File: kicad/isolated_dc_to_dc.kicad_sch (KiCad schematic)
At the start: 23 parts, among them U1001 LM25184NGUR, U1002 750313445

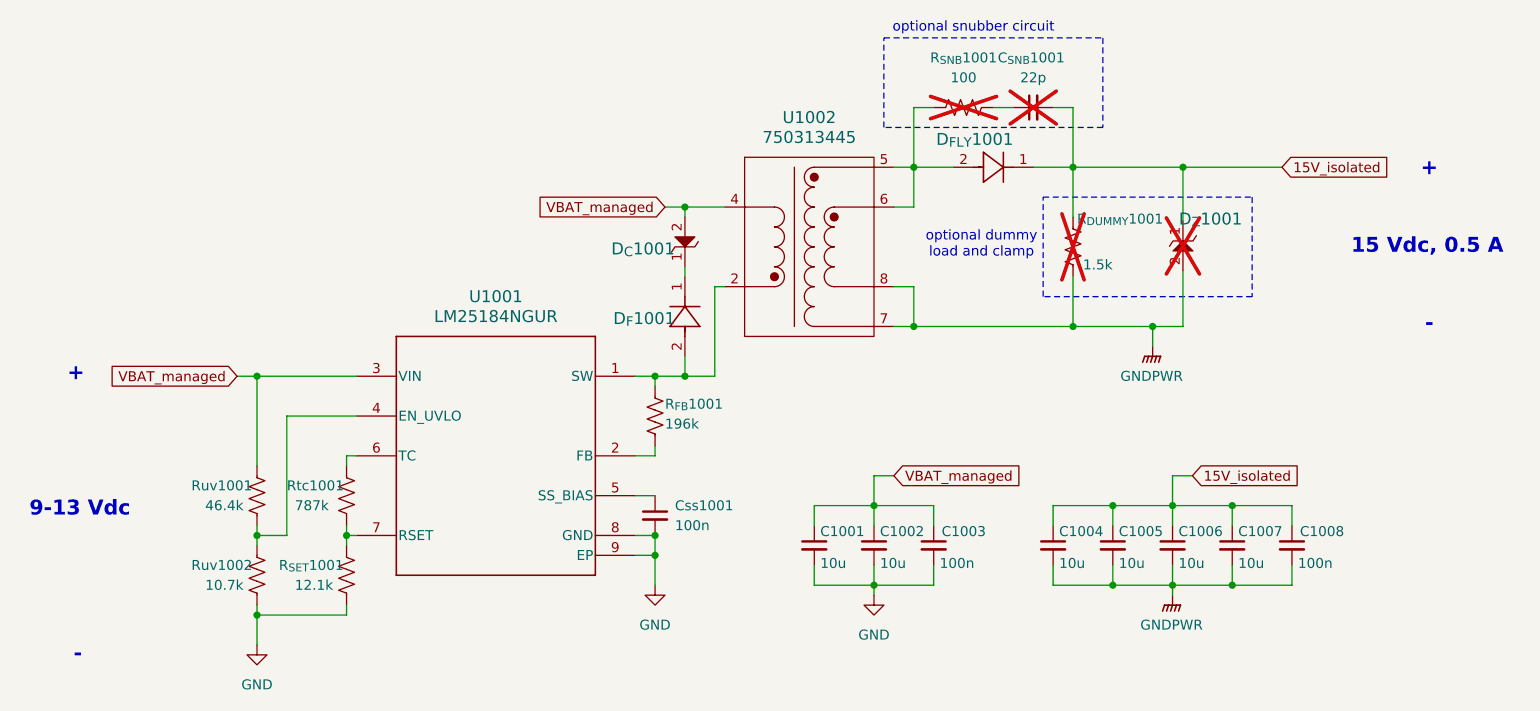
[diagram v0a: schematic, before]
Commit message: kicad
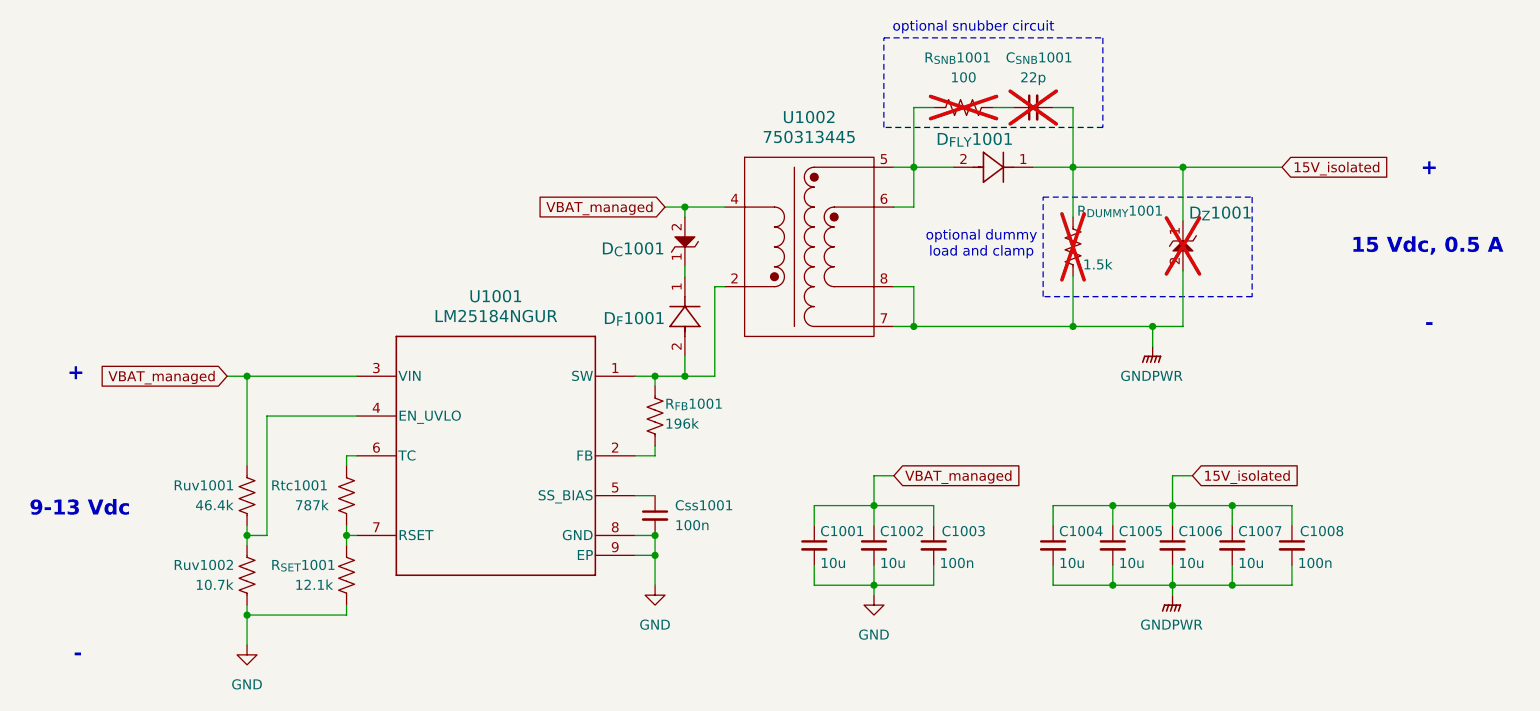
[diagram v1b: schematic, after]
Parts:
- D_{C}1001, D_{Z}1001: footprint zener_PDZVTR9.1B:DIO_PDZVTFT_ROM -> DIO_PDZVTFT_ROM
- D_{FLY}1001, D_{F}1001: footprint schottky_SK510A-LTP:SMADO-214AC_LEAD-FRAME_MCC -> SMADO-214AC_LEAD-FRAME_MCC
- U1001: footprint dc_to_dc_LM25184NGUR:NGU0008C-IPC_A -> NGU0008C-IPC_A
- U1002: footprint transformer_750313445:SOIC_13445_WRE -> SOIC_13445_WRE
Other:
- moved on the sheet: Ruv1001, Ruv1002
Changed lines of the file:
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@@
 	(paper "A4")
-	(junction
-		(at 109.22 96.52)
-		(diameter 0)
-		(color 0 0 0 0)
-	)
-	(junction
-		(at 109.22 66.04)
-		(diameter 0)
-		(color 0 0 0 0)
-	)
 	(junction
 		(at 233.68 92.71)
@@
 	)
 	(junction
+		(at 107.95 96.52)
+		(diameter 0)
+		(color 0 0 0 0)
+	)
+	(junction
 		(at 227.3899 39.37)
+		(diameter 0)
+		(color 0 0 0 0)
+	)
+	(junction
+		(at 107.95 66.04)
 		(diameter 0)
 		(color 0 0 0 0)
@@
 	)
 	(junction
-		(at 109.22 86.36)
-		(diameter 0)
-		(color 0 0 0 0)
-	)
-	(junction
 		(at 187.96 92.71)
 		(diameter 0)
@@
 	)
 	(junction
+		(at 107.95 86.36)
+		(diameter 0)
+		(color 0 0 0 0)
+	)
+	(junction
 		(at 160.02 86.36)
 		(diameter 0)
@@
 	(wire
 		(pts
-			(xy 113.03 86.36) (xy 109.22 86.36)
-		)
-		(stroke
-			(width 0)
-			(type default)
-		)
-	)
-	(wire
-		(pts
 			(xy 160.02 67.31) (xy 160.02 66.04)
 		)
@@
 	(wire
 		(pts
-			(xy 109.22 66.04) (xy 121.92 66.04)
+			(xy 107.95 96.52) (xy 120.65 96.52)
 		)
 		(stroke
@@
 	(wire
 		(pts
-			(xy 113.03 71.12) (xy 113.03 86.36)
-		)
-		(stroke
-			(width 0)
-			(type default)
-		)
-	)
-	(wire
-		(pts
-			(xy 109.22 85.09) (xy 109.22 86.36)
+			(xy 110.49 71.12) (xy 110.49 86.36)
+		)
+		(stroke
+			(width 0)
+			(type default)
+		)
+	)
+	(wire
+		(pts
+			(xy 107.95 85.09) (xy 107.95 86.36)
 		)
 		(stroke
@@
 	(wire
 		(pts
-			(xy 109.22 96.52) (xy 109.22 100.33)
+			(xy 107.95 96.52) (xy 107.95 100.33)
 		)
 		(stroke
@@
 	(wire
 		(pts
+			(xy 107.95 86.36) (xy 110.49 86.36)
+		)
+		(stroke
+			(width 0)
+			(type default)
+		)
+	)
+	(wire
+		(pts
 			(xy 157.48 76.2) (xy 160.02 76.2)
 		)
@@
 	(wire
 		(pts
-			(xy 109.22 96.52) (xy 120.65 96.52)
-		)
-		(stroke
-			(width 0)
-			(type default)
-		)
-	)
-	(wire
-		(pts
 			(xy 241.3 85.09) (xy 241.3 82.55)
 		)
@@
 	(wire
 		(pts
-			(xy 109.22 66.04) (xy 109.22 77.47)
+			(xy 107.95 66.04) (xy 107.95 77.47)
 		)
 		(stroke
@@
 	(wire
 		(pts
-			(xy 106.68 66.04) (xy 109.22 66.04)
+			(xy 105.41 66.04) (xy 107.95 66.04)
 		)
 		(stroke
@@
 	(wire
 		(pts
-			(xy 109.22 95.25) (xy 109.22 96.52)
+			(xy 107.95 95.25) (xy 107.95 96.52)
 		)
 		(stroke
@@
 	(wire
 		(pts
+			(xy 107.95 66.04) (xy 121.92 66.04)
+		)
+		(stroke
+			(width 0)
+			(type default)
+		)
+	)
+	(wire
+		(pts
 			(xy 213.36 45.72) (xy 213.36 39.37)
 		)
@@
 	(wire
 		(pts
-			(xy 121.92 71.12) (xy 113.03 71.12)
+			(xy 121.92 71.12) (xy 110.49 71.12)
 		)
 		(stroke
@@
 	(wire
 		(pts
-			(xy 109.22 86.36) (xy 109.22 87.63)
+			(xy 107.95 86.36) (xy 107.95 87.63)
 		)
 		(stroke
@@
 	(global_label "VBAT_managed"
 		(shape input)
-		(at 106.68 66.04 180)
+		(at 105.41 66.04 180)
 		(fields_autoplaced yes)
 		(effects
@@
 		)
 		(property "Intersheetrefs" "${INTERSHEET_REFS}"
-			(at 89.7855 66.04 0)
+			(at 88.5155 66.04 0)
 			(effects
 				(font
@@
 	(symbol
 		(lib_id "Device:R_US")
-		(at 109.22 81.28 0)
+		(at 107.95 81.28 0)
 		(unit 1)
 		(exclude_from_sim no)
@@
 		(dnp no)
 		(property "Reference" "Ruv1001"
-			(at 100.838 80.01 0)
+			(at 98.552 80.01 0)
 			(effects
 				(font
@@
 		)
 		(property "Value" "46.4k"
-			(at 102.616 82.55 0)
+			(at 101.346 82.55 0)
 			(effects
 				(font
@@
 		)
 		(property "Footprint" "Resistor_SMD:R_0402_1005Metric"
-			(at 110.236 81.534 90)
+			(at 108.966 81.534 90)
 			(effects
 				(font
@@
 		)
 		(property "Datasheet" "~"
-			(at 109.22 81.28 0)
+			(at 107.95 81.28 0)
 			(effects
 				(font
@@
 		)
 		(property "Description" "Resistor, US symbol"
-			(at 109.22 81.28 0)
+			(at 107.95 81.28 0)
 			(effects
 				(font
@@
 		(on_board yes)
 		(dnp yes)
-		(fields_autoplaced yes)
 		(property "Reference" "R_{SNB}1001"
-			(at 199.39 25.4 90)
+			(at 198.628 25.4 90)
 			(effects
 				(font
@@
 	)
 	(symbol
-		(lib_name "PDZVTR9.1B_1")
 		(lib_id "zener_PDZVTR9.1B:PDZVTR9.1B")
 		(at 227.3899 46.2395 270)
@@
 		(dnp yes)
 		(property "Reference" "D_{Z}1001"
-			(at 234.95 45.974 90)
+			(at 236.22 45.212 90)
 			(effects
 				(font
@@
 			)
 		)
-		(property "Footprint" "zener_PDZVTR9.1B:DIO_PDZVTFT_ROM"
+		(property "Footprint" "DIO_PDZVTFT_ROM"
 			(at 236.5339 36.0795 0)
 			(effects
@@
 			)
 		)
-		(property "Footprint" "schottky_SK510A-LTP:SMADO-214AC_LEAD-FRAME_MCC"
+		(property "Footprint" "SMADO-214AC_LEAD-FRAME_MCC"
 			(at 198.12 39.37 0)
 			(effects
@@
 		(dnp yes)
 		(property "Reference" "R_{DUMMY}1001"
-			(at 213.868 45.974 0)
+			(at 213.868 44.958 0)
 			(effects
 				(font
@@
 		(dnp no)
 		(property "Reference" "Rtc1001"
-			(at 113.03 80.01 0)
+			(at 110.998 80.01 0)
 			(effects
 				(font
@@
 		(dnp yes)
 		(property "Reference" "C_{SNB}1001"
-			(at 208.026 25.4 90)
+			(at 209.042 25.4 90)
 			(effects
 				(font
@@
 		(dnp no)
 		(property "Reference" "R_{SET}1001"
-			(at 112.014 90.17 0)
+			(at 110.998 90.17 0)
 			(effects
 				(font
@@
 		(dnp no)
 		(property "Reference" "D_{F}1001"
-			(at 154.686 58.674 90)
+			(at 153.416 58.674 90)
 			(effects
 				(font
@@
 			)
 		)
-		(property "Footprint" "schottky_SK510A-LTP:SMADO-214AC_LEAD-FRAME_MCC"
+		(property "Footprint" "SMADO-214AC_LEAD-FRAME_MCC"
 			(at 163.83 63.5 0)
 			(effects
@@
 	(symbol
 		(lib_id "Device:R_US")
-		(at 109.22 91.44 0)
+		(at 107.95 91.44 0)
 		(unit 1)
 		(exclude_from_sim no)
@@
 		(dnp no)
 		(property "Reference" "Ruv1002"
-			(at 100.838 90.17 0)
+			(at 98.552 90.17 0)
 			(effects
 				(font
@@
 		)
 		(property "Value" "10.7k"
-			(at 102.616 92.71 0)
+			(at 101.346 92.71 0)
 			(effects
 				(font
@@
 		)
 		(property "Footprint" "Resistor_SMD:R_0402_1005Metric"
-			(at 110.236 91.694 90)
+			(at 108.966 91.694 90)
 			(effects
 				(font
@@
 		)
 		(property "Datasheet" "~"
-			(at 109.22 91.44 0)
+			(at 107.95 91.44 0)
 			(effects
 				(font
@@
 		)
 		(property "Description" "Resistor, US symbol"
-			(at 109.22 91.44 0)
+			(at 107.95 91.44 0)
 			(effects
 				(font
@@
 	)
 	(symbol
-		(lib_name "PDZVTR9.1B_1")
 		(lib_id "zener_PDZVTR9.1B:PDZVTR9.1B")
 		(at 163.83 52.07 90)
@@
 		(dnp no)
 		(property "Reference" "D_{C}1001"
-			(at 154.432 49.784 90)
+			(at 153.162 49.784 90)
 			(effects
 				(font
@@
 			)
 		)
-		(property "Footprint" "zener_PDZVTR9.1B:DIO_PDZVTFT_ROM"
+		(property "Footprint" "DIO_PDZVTFT_ROM"
 			(at 154.686 62.23 0)
 			(effects
@@
 	)
 	(symbol
-		(lib_name "750313445_1")
 		(lib_id "transformer_750313445:750313445")
 		(at 168.91 44.45 0)
@@
 			)
 		)
-		(property "Footprint" "transformer_750313445:SOIC_13445_WRE"
+		(property "Footprint" "SOIC_13445_WRE"
 			(at 161.798 31.496 0)
 			(effects
@@
 	(symbol
 		(lib_id "power:GND")
-		(at 109.22 100.33 0)
+		(at 107.95 100.33 0)
 		(unit 1)
 		(exclude_from_sim no)
@@
 		(fields_autoplaced yes)
 		(property "Reference" "#PWR01001"
-			(at 109.22 106.68 0)
+			(at 107.95 106.68 0)
 			(effects
 				(font
@@
 		)
 		(property "Value" "GND"
-			(at 109.22 105.41 0)
+			(at 107.95 105.41 0)
 			(effects
 				(font
@@
 		)
 		(property "Footprint" ""
-			(at 109.22 100.33 0)
+			(at 107.95 100.33 0)
 			(effects
 				(font
@@
 		)
 		(property "Datasheet" ""
-			(at 109.22 100.33 0)
+			(at 107.95 100.33 0)
 			(effects
 				(font
@@
 		)
 		(property "Description" "Power symbol creates a global label with name \"GND\" , ground"
-			(at 109.22 100.33 0)
+			(at 107.95 100.33 0)
 			(effects
 				(font
@@
 			)
 		)
-		(property "Footprint" "dc_to_dc_LM25184NGUR:NGU0008C-IPC_A"
+		(property "Footprint" "NGU0008C-IPC_A"
 			(at 120.142 57.404 0)
 			(effects

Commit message: kicad
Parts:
- D_{C}1001, D_{Z}1001: footprint DIO_PDZVTFT_ROM -> zener_PDZVTR9.1B:DIO_PDZVTFT_ROM
- D_{FLY}1001, D_{F}1001: footprint SMADO-214AC_LEAD-FRAME_MCC -> schottky_SK510A-LTP:SMADO-214AC_LEAD-FRAME_MCC
- U1001: footprint NGU0008C-IPC_A -> dc_to_dc_LM25184NGUR:NGU0008C-IPC_A
- U1002: footprint SOIC_13445_WRE -> transformer_750313445:SOIC_13445_WRE
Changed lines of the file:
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@@
 			)
 		)
-		(property "Footprint" "DIO_PDZVTFT_ROM"
+		(property "Footprint" "zener_PDZVTR9.1B:DIO_PDZVTFT_ROM"
 			(at 236.5339 36.0795 0)
 			(effects
@@
 			)
 		)
-		(property "Footprint" "SMADO-214AC_LEAD-FRAME_MCC"
+		(property "Footprint" "schottky_SK510A-LTP:SMADO-214AC_LEAD-FRAME_MCC"
 			(at 198.12 39.37 0)
 			(effects
@@
 			)
 		)
-		(property "Footprint" "SMADO-214AC_LEAD-FRAME_MCC"
+		(property "Footprint" "schottky_SK510A-LTP:SMADO-214AC_LEAD-FRAME_MCC"
 			(at 163.83 63.5 0)
 			(effects
@@
 			)
 		)
-		(property "Footprint" "DIO_PDZVTFT_ROM"
+		(property "Footprint" "zener_PDZVTR9.1B:DIO_PDZVTFT_ROM"
 			(at 154.686 62.23 0)
 			(effects
@@
 			)
 		)
-		(property "Footprint" "SOIC_13445_WRE"
+		(property "Footprint" "transformer_750313445:SOIC_13445_WRE"
 			(at 161.798 31.496 0)
 			(effects
@@
 			)
 		)
-		(property "Footprint" "NGU0008C-IPC_A"
+		(property "Footprint" "dc_to_dc_LM25184NGUR:NGU0008C-IPC_A"
 			(at 120.142 57.404 0)
 			(effects
